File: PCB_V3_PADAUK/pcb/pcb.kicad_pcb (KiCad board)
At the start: 2 copper layers, 54.6 x 26.7 mm, 41 parts, among them J1 FLUSH_SWITCH, J3 BATTERY, J4 SOLENOID, J5 BUZZER_CONN, J6 L_DETECT, J7 Programming Connector, Q1 DMG2301L, Q2 BC817, Q3 BC817, Q4 DMG2301L, U1 PMS171B, U2 AZ1117-1.8, U3 DRV8837, Y1 32khz_smd, Y2 32khz_th

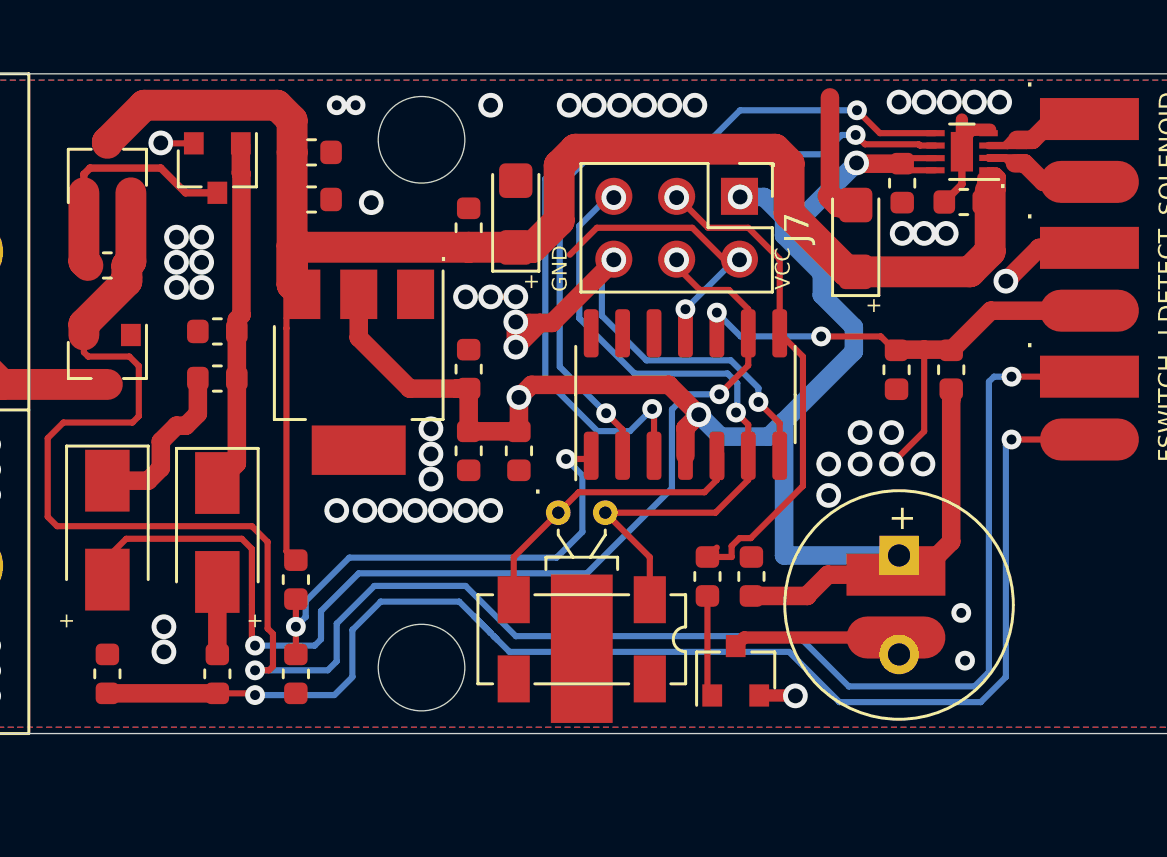
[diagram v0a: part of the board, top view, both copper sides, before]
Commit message: Add files via upload
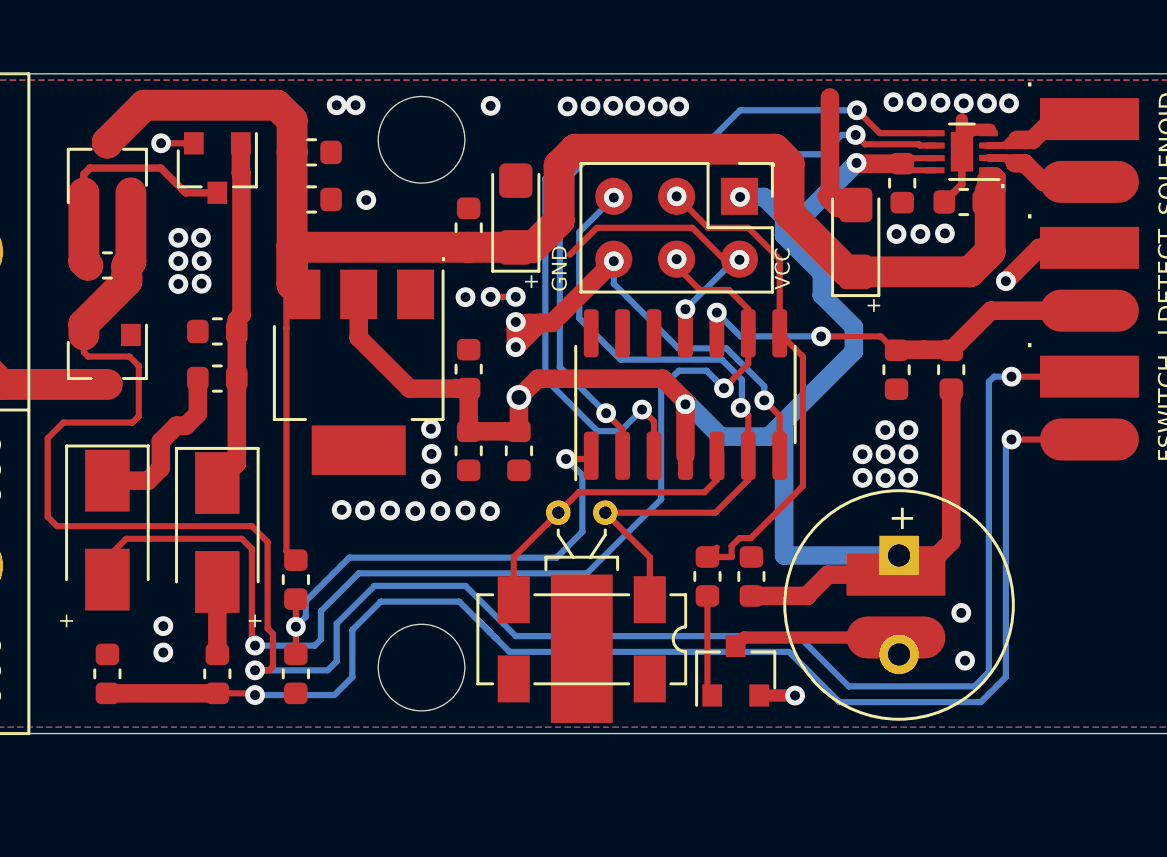
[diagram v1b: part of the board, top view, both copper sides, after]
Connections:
- J7 pad 6: Net-(J7-Pad6) -> GND
- U1 pad 7: Net-(J7-Pad6) -> GND
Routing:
- net Net-(J7-Pad6): track 21.5 -> 0.00 mm, vias 4 -> 0
- net GND: track 30.2 -> 50.4 mm, vias 64 -> 71
- net L_DETECT: track 21.4 -> 16.1 mm, vias 3 -> 2
- net POWER_CONTROL: track 44.5 -> 45.8 mm
